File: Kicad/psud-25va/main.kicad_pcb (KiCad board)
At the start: 2 copper layers, 125 x 60 mm, 57 parts, among them K1 MAIN AC, K2 PSU1, K3 PSU2, X101 LOGO

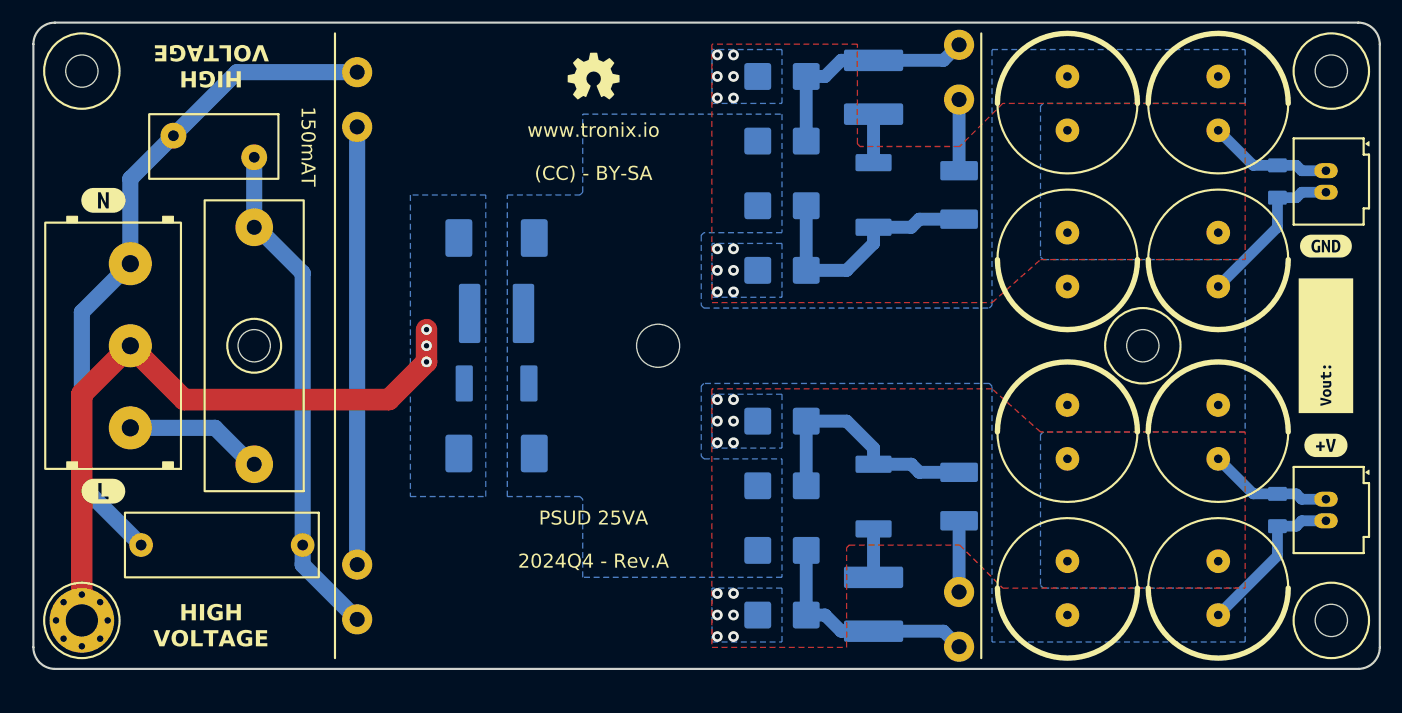
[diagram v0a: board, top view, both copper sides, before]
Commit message: Up
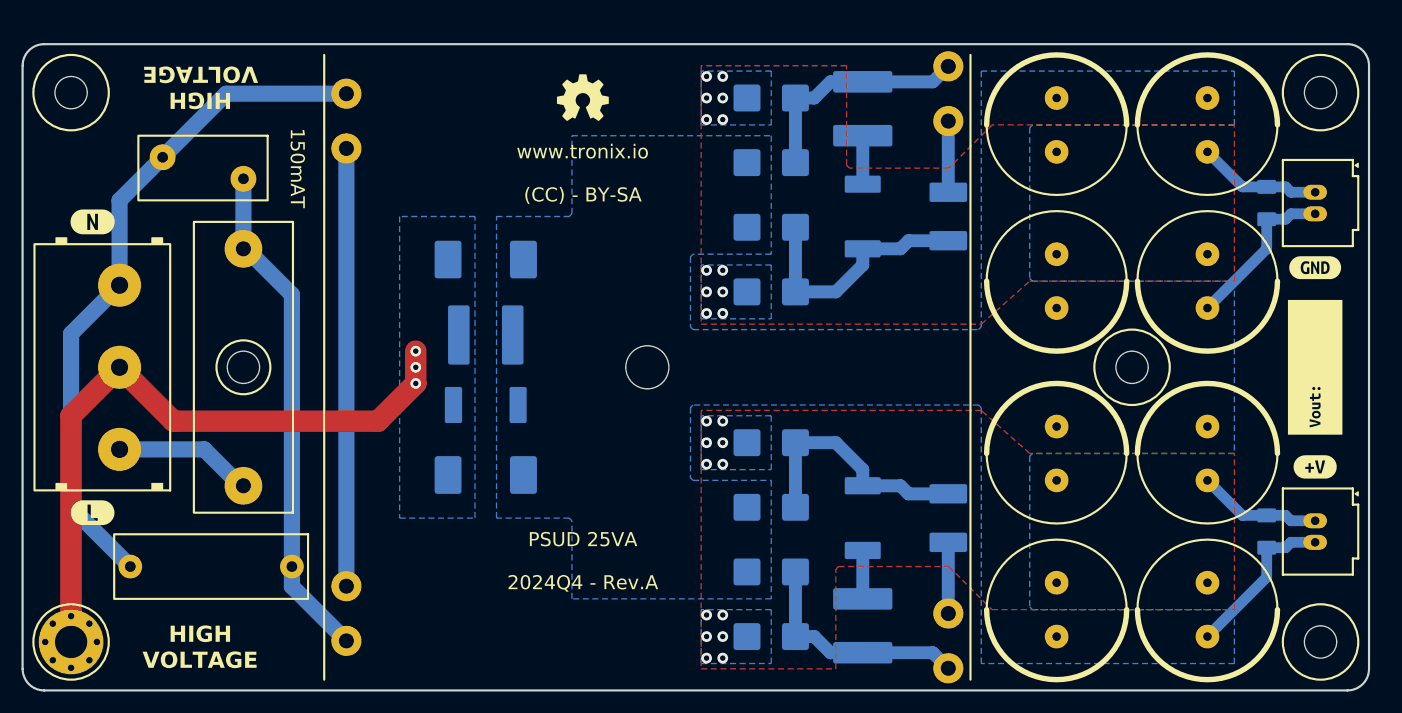
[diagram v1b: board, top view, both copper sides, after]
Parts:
- moved C1 2.24 mm to (102.5, 108.5)
- moved C10 2.24 mm to (195.0, 82.0)
- moved C11 2.24 mm to (195.0, 98.0)
- moved C12 2.24 mm to (200.5, 74.8)
- moved C13 2.24 mm to (200.5, 105.2)
- moved C14 2.24 mm to (128.0, 87.0)
- moved C2 2.24 mm to (163.0, 66.0)
- moved C3 2.24 mm to (163.0, 114.0)
- moved C4 2.24 mm to (181.0, 67.5)
- moved C5 2.24 mm to (181.0, 112.5)
- moved C6 2.24 mm to (181.0, 82.0)
- moved C7 2.24 mm to (181.0, 98.0)
- moved C8 2.24 mm to (195.0, 67.5)
- moved C9 2.24 mm to (195.0, 112.5)
- moved D1 2.24 mm to (154.5, 83.0)
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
